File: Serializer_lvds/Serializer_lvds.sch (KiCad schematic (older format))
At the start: 32 parts, among them U1 plot_v1, U10 adc_bridge_6, U11 adc_bridge_6, U12 plot_v1, U13 madhuri_buffer, U14 plot_v1, U15 plot_v1, U16 plot_v1, U17 dac_bridge_2, U18 plot_v1, U19 plot_v1, U2 madhuri_piso, U20 plot_v1, U3 plot_v1, U4 plot_v1, U5 plot_v1, U6 plot_v1, U7 plot_v1, U8 plot_v1, U9 plot_v1, X1 LVDS_Drvr

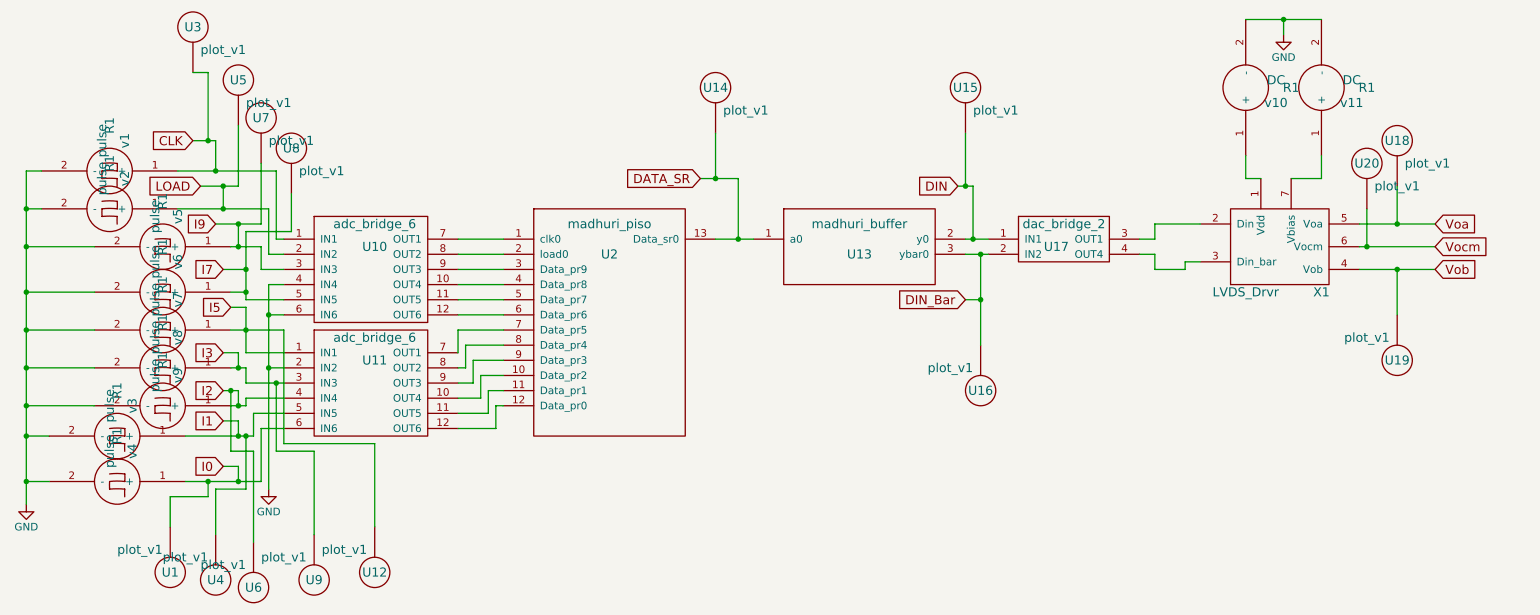
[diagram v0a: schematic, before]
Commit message: new files update
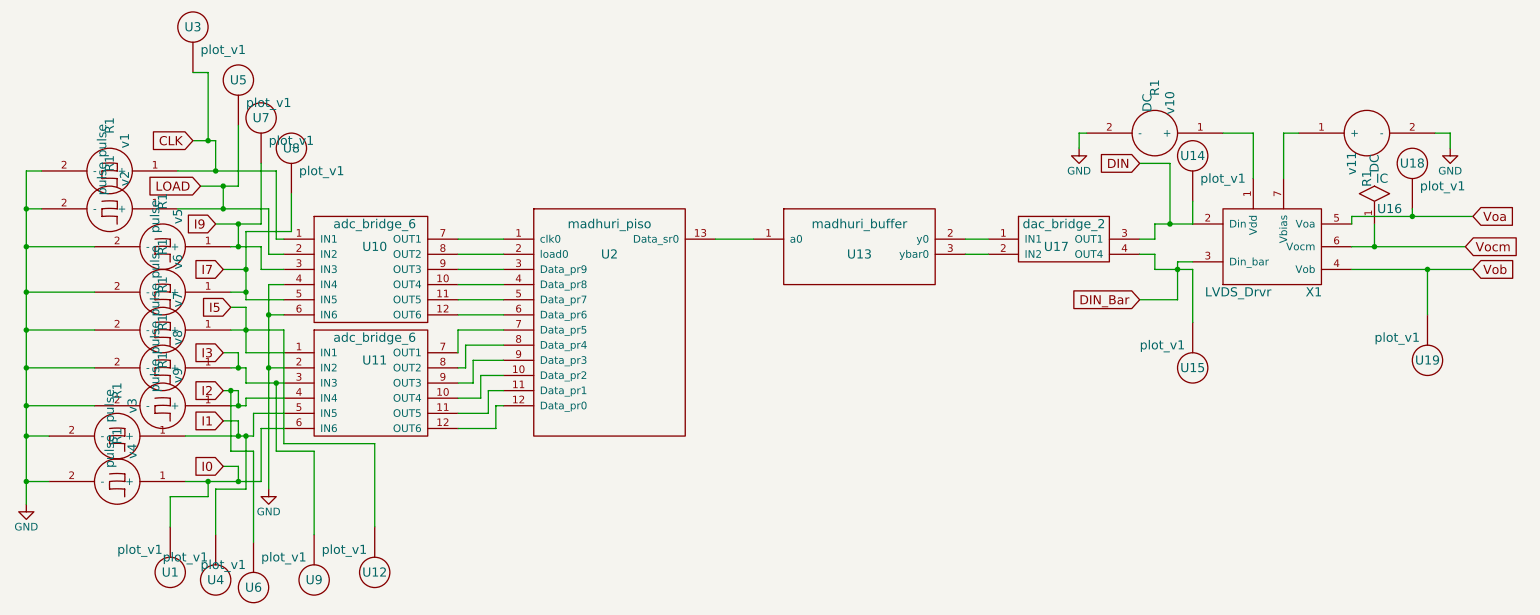
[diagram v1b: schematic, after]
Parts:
- removed U16, U20: plot_v1, symbol plot_v1
- added U16: IC, symbol IC
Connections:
- net DIN: now also U14.~, U17.3 (OUT1), X1.2 (Din); no longer U13.2 (y0), U15.~, U17.1 (IN1)
- net DIN_Bar: now also U15.~, U17.4 (OUT4), X1.3 (Din_bar); no longer U13.3 (ybar0), U17.2 (IN2)
- net Vocm: now also U16.1
- net DATA_SR: no longer names the net of U13.1 (a0), U2.13 (Data_sr0)
- net DATA_SR: no longer U14.~
- new net: U13.2 (y0), U17.1 (IN1)
- new net: U13.3 (ybar0), U17.2 (IN2)
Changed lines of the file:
@@
 EESchema Schematic File Version 2
+LIBS:Serializer_lvds-rescue
 LIBS:adc-dac
 LIBS:memory
@@
 $EndComp
 $Comp
-L DC v10
-U 1 1 62297F4D
-P 9250 1700
-F 0 "v10" H 9050 1800 60  0000 C CNN
-F 1 "DC" H 9050 1650 60  0000 C CNN
-F 2 "R1" H 8950 1700 60  0000 C CNN
-F 3 "" H 9250 1700 60  0000 C CNN
-	1    9250 1700
-	-1   0    0    1
-$EndComp
-$Comp
-L DC v11
-U 1 1 62297FC0
-P 9750 1700
-F 0 "v11" H 9550 1800 60  0000 C CNN
-F 1 "DC" H 9550 1650 60  0000 C CNN
-F 2 "R1" H 9450 1700 60  0000 C CNN
-F 3 "" H 9750 1700 60  0000 C CNN
-	1    9750 1700
-	-1   0    0    1
-$EndComp
-$Comp
-L GND #PWR01
-U 1 1 62298019
-P 9500 1350
-F 0 "#PWR01" H 9500 1100 50  0001 C CNN
-F 1 "GND" H 9500 1200 50  0000 C CNN
-F 2 "" H 9500 1350 50  0001 C CNN
-F 3 "" H 9500 1350 50  0001 C CNN
-	1    9500 1350
-	1    0    0    -1
-$EndComp
-$Comp
 L pulse v1
 U 1 1 6229813E
@@
 $EndComp
 $Comp
-L GND #PWR02
+L GND #PWR2
 U 1 1 62298923
 P 2800 4350
-F 0 "#PWR02" H 2800 4100 50  0001 C CNN
+F 0 "#PWR2" H 2800 4100 50  0001 C CNN
 F 1 "GND" H 2800 4200 50  0000 C CNN
 F 2 "" H 2800 4350 50  0001 C CNN
@@
 $EndComp
 $Comp
-L GND #PWR03
+L GND #PWR1
 U 1 1 62298959
 P 1200 4450
-F 0 "#PWR03" H 1200 4200 50  0001 C CNN
+F 0 "#PWR1" H 1200 4200 50  0001 C CNN
 F 1 "GND" H 1200 4300 50  0000 C CNN
 F 2 "" H 1200 4450 50  0001 C CNN
@@
 	1    0    0    -1
 $EndComp
-Text GLabel 10500 2600 2    60   Input ~ 0
-Voa
-Text GLabel 10500 2900 2    60   Input ~ 0
-Vob
 Text GLabel 2300 2050 0    60   Input ~ 0
 CLK
@@
 Text GLabel 2500 4200 0    60   Input ~ 0
 I0
-Text GLabel 5650 2300 0    60   Input ~ 0
-DATA_SR
-Text GLabel 7350 2350 0    60   Input ~ 0
+Text GLabel 8550 2200 0    60   Input ~ 0
 DIN
-Text GLabel 7400 3100 0    60   Input ~ 0
+Text GLabel 8550 3100 0    60   Input ~ 0
 DIN_Bar
 $Comp
@@
 	8650 2700 8650 2600
 Wire Wire Line
-	8650 2600 8950 2600
-Wire Wire Line
 	8550 2800 8650 2800
 Wire Wire Line
 	8650 2800 8650 2900
-Wire Wire Line
-	8650 2900 8850 2900
-Wire Wire Line
-	9250 2150 9250 2300
-Wire Wire Line
-	9750 2150 9750 2300
-Wire Wire Line
-	9250 1250 9750 1250
-Wire Wire Line
-	9500 1250 9500 1350
-Connection ~ 9500 1250
 Wire Wire Line
 	2200 2250 2850 2250
@@
 Connection ~ 1200 2500
 Wire Wire Line
-	10000 2600 10500 2600
-Wire Wire Line
-	10000 2900 10500 2900
-Wire Wire Line
 	2300 2050 2450 2050
 Wire Wire Line
@@
 	2600 4200 2600 4300
 Connection ~ 2600 4300
-Wire Wire Line
-	5650 2300 5900 2300
-Wire Wire Line
-	5900 2300 5900 2700
-Connection ~ 5900 2700
-Wire Wire Line
-	7350 2350 7450 2350
-Wire Wire Line
-	7450 2350 7450 2700
-Connection ~ 7450 2700
-Wire Wire Line
-	7400 3100 7500 3100
-Wire Wire Line
-	7500 2800 7500 3400
-Connection ~ 7500 2800
 Wire Wire Line
 	2300 1600 2400 1600
@@
 	2900 4050 2900 3300
 $Comp
+L LVDS_Drvr X1
+U 1 1 62373A6B
+P 9450 2900
+F 0 "X1" H 9700 2750 60  0000 C CNN
+F 1 "LVDS_Drvr" H 9200 2750 60  0000 C CNN
+F 2 "" H 9450 2900 60  0001 C CNN
+F 3 "" H 9450 2900 60  0001 C CNN
+	1    9450 2900
+	1    0    0    -1
+$EndComp
+Wire Wire Line
+	8650 2600 8900 2600
+Wire Wire Line
+	8650 2900 8900 2900
+Wire Wire Line
+	8800 2850 8800 3100
+Wire Wire Line
+	8800 2850 8900 2850
+$Comp
+L DC v10
+U 1 1 62373D44
+P 8650 2000
+F 0 "v10" H 8450 2100 60  0000 C CNN
+F 1 "DC" H 8450 1950 60  0000 C CNN
+F 2 "R1" H 8350 2000 60  0000 C CNN
+F 3 "" H 8650 2000 60  0000 C CNN
+	1    8650 2000
+	0    1    1    0
+$EndComp
+$Comp
+L DC v11
+U 1 1 62373DB1
+P 10050 2000
+F 0 "v11" H 9850 2100 60  0000 C CNN
+F 1 "DC" H 9850 1950 60  0000 C CNN
+F 2 "R1" H 9750 2000 60  0000 C CNN
+F 3 "" H 10050 2000 60  0000 C CNN
+	1    10050 2000
+	0    -1   -1   0
+$EndComp
+Wire Wire Line
+	9100 2000 9300 2000
+Wire Wire Line
+	9300 2000 9300 2300
+Wire Wire Line
+	9600 2000 9500 2000
+Wire Wire Line
+	9500 2000 9500 2300
+$Comp
+L GND #PWR3
+U 1 1 62373FCE
+P 8150 2100
+F 0 "#PWR3" H 8150 1850 50  0001 C CNN
+F 1 "GND" H 8150 1950 50  0000 C CNN
+F 2 "" H 8150 2100 50  0001 C CNN
+F 3 "" H 8150 2100 50  0001 C CNN
+	1    8150 2100
+	1    0    0    -1
+$EndComp
+$Comp
+L GND #PWR4
+U 1 1 62374016
+P 10600 2100
+F 0 "#PWR4" H 10600 1850 50  0001 C CNN
+F 1 "GND" H 10600 1950 50  0000 C CNN
+F 2 "" H 10600 2100 50  0001 C CNN
+F 3 "" H 10600 2100 50  0001 C CNN
+	1    10600 2100
+	1    0    0    -1
+$EndComp
+Wire Wire Line
+	8200 2000 8150 2000
+Wire Wire Line
+	8150 2000 8150 2100
+Wire Wire Line
+	10500 2000 10600 2000
+Wire Wire Line
+	10600 2000 10600 2100
+Text GLabel 10750 2550 2    60   Input ~ 0
+Voa
+Text GLabel 10750 2900 2    60   Input ~ 0
+Vob
+Wire Wire Line
+	10750 2550 9950 2550
+Wire Wire Line
+	9950 2550 9950 2600
+Wire Wire Line
+	9950 2900 10750 2900
+Wire Wire Line
+	8550 2200 8750 2200
+Wire Wire Line
+	8750 2200 8750 2600
+Connection ~ 8750 2600
+Wire Wire Line
+	8800 3100 8550 3100
+Connection ~ 8800 2900
+$Comp
 L plot_v1 U14
-U 1 1 6229ACD5
-P 5750 2200
-F 0 "U14" H 5750 2700 60  0000 C CNN
-F 1 "plot_v1" H 5950 2550 60  0000 C CNN
-F 2 "" H 5750 2200 60  0000 C CNN
-F 3 "" H 5750 2200 60  0000 C CNN
-	1    5750 2200
+U 1 1 6237451D
+P 8900 2650
+F 0 "U14" H 8900 3150 60  0000 C CNN
+F 1 "plot_v1" H 9100 3000 60  0000 C CNN
+F 2 "" H 8900 2650 60  0000 C CNN
+F 3 "" H 8900 2650 60  0000 C CNN
+	1    8900 2650
 	1    0    0    -1
 $EndComp
 $Comp
 L plot_v1 U15
-U 1 1 6229AD4C
-P 7400 2200
-F 0 "U15" H 7400 2700 60  0000 C CNN
-F 1 "plot_v1" H 7600 2550 60  0000 C CNN
-F 2 "" H 7400 2200 60  0000 C CNN
-F 3 "" H 7400 2200 60  0000 C CNN
-	1    7400 2200
-	1    0    0    -1
-$EndComp
-$Comp
-L plot_v1 U16
-U 1 1 6229ADDB
-P 7500 3200
-F 0 "U16" H 7500 3700 60  0000 C CNN
-F 1 "plot_v1" H 7700 3550 60  0000 C CNN
-F 2 "" H 7500 3200 60  0000 C CNN
-F 3 "" H 7500 3200 60  0000 C CNN
-	1    7500 3200
+U 1 1 623745A6
+P 8900 3050
+F 0 "U15" H 8900 3550 60  0000 C CNN
+F 1 "plot_v1" H 9100 3400 60  0000 C CNN
+F 2 "" H 8900 3050 60  0000 C CNN
+F 3 "" H 8900 3050 60  0000 C CNN
+	1    8900 3050
 	-1   0    0    1
 $EndComp
 $Comp
 L plot_v1 U18
-U 1 1 6229AE76
-P 10250 2550
-F 0 "U18" H 10250 3050 60  0000 C CNN
-F 1 "plot_v1" H 10450 2900 60  0000 C CNN
-F 2 "" H 10250 2550 60  0000 C CNN
-F 3 "" H 10250 2550 60  0000 C CNN
-	1    10250 2550
+U 1 1 62374637
+P 10350 2700
+F 0 "U18" H 10350 3200 60  0000 C CNN
+F 1 "plot_v1" H 10550 3050 60  0000 C CNN
+F 2 "" H 10350 2700 60  0000 C CNN
+F 3 "" H 10350 2700 60  0000 C CNN
+	1    10350 2700
 	1    0    0    -1
 $EndComp
 $Comp
 L plot_v1 U19
-U 1 1 6229AF33
-P 10250 3000
-F 0 "U19" H 10250 3500 60  0000 C CNN
-F 1 "plot_v1" H 10450 3350 60  0000 C CNN
-F 2 "" H 10250 3000 60  0000 C CNN
-F 3 "" H 10250 3000 60  0000 C CNN
-	1    10250 3000
+U 1 1 6237469E
+P 10450 3000
+F 0 "U19" H 10450 3500 60  0000 C CNN
+F 1 "plot_v1" H 10650 3350 60  0000 C CNN
+F 2 "" H 10450 3000 60  0000 C CNN
+F 3 "" H 10450 3000 60  0000 C CNN
+	1    10450 3000
 	-1   0    0    1
 $EndComp
 Wire Wire Line
-	5750 2000 5750 2300
-Connection ~ 5750 2300
-Wire Wire Line
-	7400 2000 7400 2350
-Connection ~ 7400 2350
-Connection ~ 7500 3100
-Wire Wire Line
-	10250 2350 10250 2600
-Connection ~ 10250 2600
-Wire Wire Line
-	10250 3200 10250 2900
-Connection ~ 10250 2900
-$Comp
-L LVDS_Drvr X1
-U 1 1 6229AB19
-P 9500 2900
-F 0 "X1" H 9750 2750 60  0000 C CNN
-F 1 "LVDS_Drvr" H 9250 2750 60  0000 C CNN
-F 2 "" H 9500 2900 60  0001 C CNN
-F 3 "" H 9500 2900 60  0001 C CNN
-	1    9500 2900
-	1    0    0    -1
-$EndComp
-Wire Wire Line
-	8950 2850 8850 2850
-Wire Wire Line
-	8850 2850 8850 2900
-Wire Wire Line
-	9250 2300 9350 2300
-Wire Wire Line
-	9750 2300 9550 2300
-Text GLabel 10500 2750 2    60   Input ~ 0
+	8900 2600 8900 2450
+Wire Wire Line
+	8900 2900 8900 3250
+Wire Wire Line
+	10350 2500 10350 2550
+Connection ~ 10350 2550
+Wire Wire Line
+	10450 3200 10450 2900
+Connection ~ 10450 2900
+Text GLabel 10700 2750 2    60   Input ~ 0
 Vocm
 Wire Wire Line
-	10500 2750 10000 2750
-$Comp
-L plot_v1 U20
-U 1 1 6229B342
-P 10050 2700
-F 0 "U20" H 10050 3200 60  0000 C CNN
-F 1 "plot_v1" H 10250 3050 60  0000 C CNN
-F 2 "" H 10050 2700 60  0000 C CNN
-F 3 "" H 10050 2700 60  0000 C CNN
-	1    10050 2700
-	1    0    0    -1
-$EndComp
-Wire Wire Line
-	10050 2500 10050 2750
-Connection ~ 10050 2750
+	9950 2750 10700 2750
+$Comp
+L IC U16
+U 1 1 62374B48
+P 9900 2650
+F 0 "U16" H 10200 2800 60  0000 C CNN
+F 1 "IC" H 10150 3000 60  0000 C CNN
+F 2 "" H 9900 2650 60  0000 C CNN
+F 3 "" H 9900 2650 60  0000 C CNN
+	1    9900 2650
+	1    0    0    -1
+$EndComp
+Wire Wire Line
+	10100 2600 10100 2750
+Connection ~ 10100 2750
 $EndSCHEMATC
